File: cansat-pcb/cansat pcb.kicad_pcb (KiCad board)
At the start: 2 copper layers, 63 x 109 mm, 21 parts, among them J1 Conn_01x02_Pin, J4 Conn_01x03_Pin, J5 Conn_01x03_Pin, J6 Conn_01x03_Pin, Q1 AO3400A, Q2 2N3904, Q3 DMG2301L, SW1 SW_DPDT_x2, U3 MPU6050, U5 SGP30

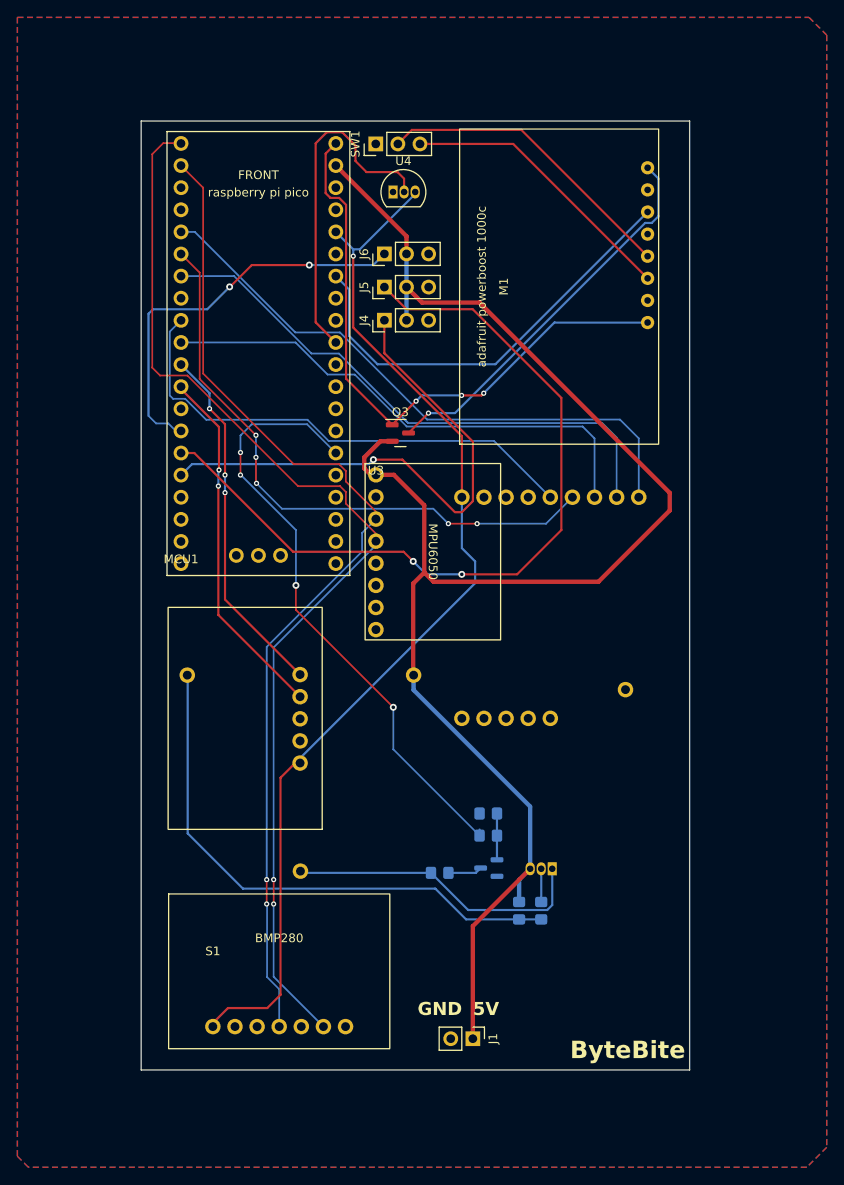
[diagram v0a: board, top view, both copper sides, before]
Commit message: V2
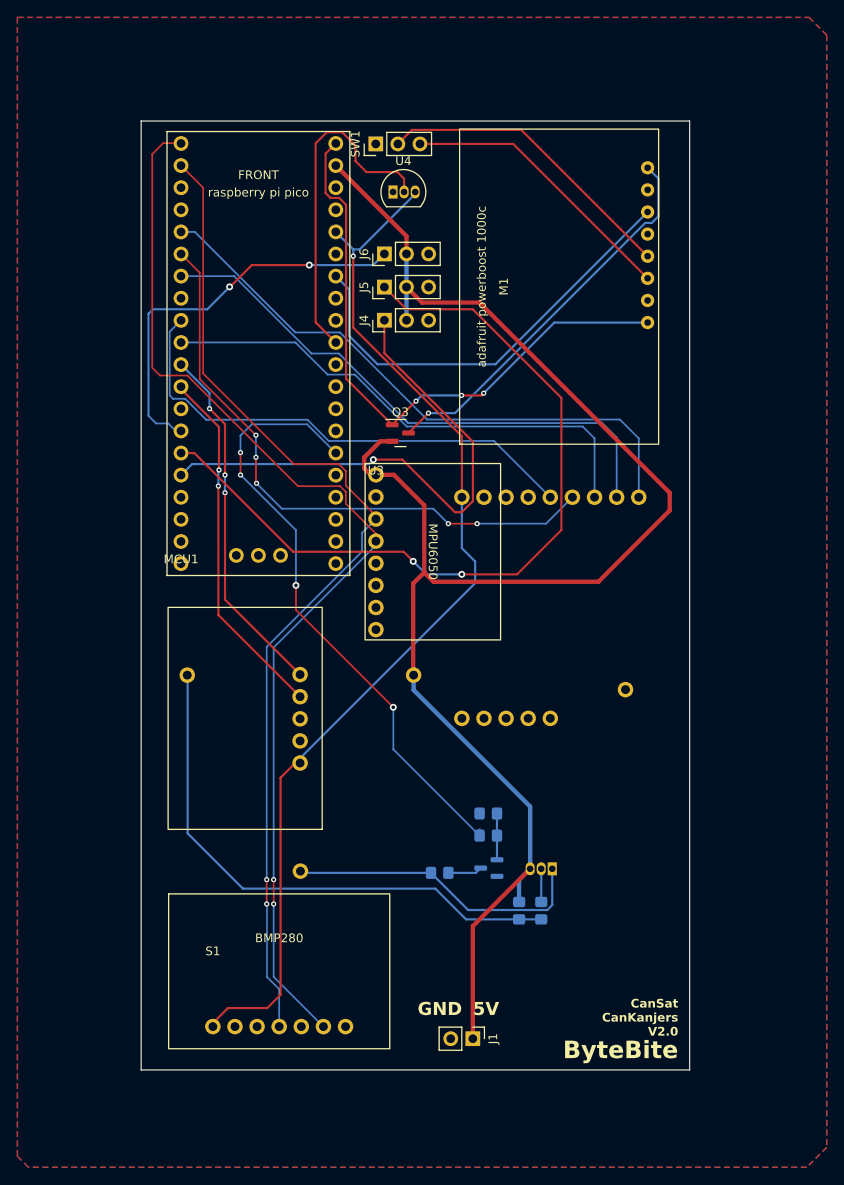
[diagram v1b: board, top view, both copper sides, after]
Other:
- board text added: "CanSat CanKanjers V2.0"
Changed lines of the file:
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@@
   (setup
     (pad_to_mask_clearance 0)
-    (grid_origin 152.14 59.58)
+    (grid_origin 177.54 135.78)
     (pcbplotparams
       (layerselection 0x00010fc_ffffffff)
@@
     (effects (font (size 1.5 1.5) (thickness 0.3) bold) (justify left bottom))
   )
-  (gr_text "ByteBite" (at 181.888 146.714) (layer "F.SilkS")
-    (effects (font (size 2 2) (thickness 0.4) bold))
+  (gr_text "CanSat\nCanKanjers\nV2.0" (at 187.7 145.178) (layer "F.SilkS")
+    (effects (font (size 1 1) (thickness 0.2) bold) (justify right bottom))
+  )
+  (gr_text "ByteBite" (at 187.7 146.714) (layer "F.SilkS")
+    (effects (font (size 2 2) (thickness 0.4) bold) (justify right))
   )
   (segment (start 152.67 78.896) (end 156.006 78.896) (width 0.25) (layer "F.Cu") (net 1))
@@
   (segment (start 158.842346 74.29) (end 180.993 74.29) (width 0.2) (layer "B.Cu") (net 20))
   (segment (start 130.58 52.734) (end 132.161686 52.734) (width 0.2) (layer "B.Cu") (net 20))
-  (segment (start 148.716346 79.404) (end 143.516 79.404) (width 0.2) (layer "F.Cu") (net 22))
-  (segment (start 149.51 80.197654) (end 148.716346 79.404) (width 0.2) (layer "F.Cu") (net 22))
-  (segment (start 149.51 81.404635) (end 152.966865 84.8615) (width 0.2) (layer "F.Cu") (net 22))
-  (segment (start 143.516 79.404) (end 133.12 69.008) (width 0.2) (layer "F.Cu") (net 22))
-  (segment (start 152.966865 84.8615) (end 152.966865 85.72) (width 0.2) (layer "F.Cu") (net 22))
-  (segment (start 149.51 80.197654) (end 149.51 81.404635) (width 0.2) (layer "F.Cu") (net 22))
-  (segment (start 133.12 69.008) (end 133.12 47.654) (width 0.2) (layer "F.Cu") (net 22))
-  (segment (start 133.12 47.654) (end 130.58 45.114) (width 0.2) (layer "F.Cu") (net 22))
+  (segment (start 149.51 81.877317) (end 152.966865 85.334182) (width 0.2) (layer "F.Cu") (net 22))
+  (segment (start 130.58 45.114) (end 133.12 47.654) (width 0.2) (layer "F.Cu") (net 22))
+  (segment (start 133.12 69.008) (end 143.516 79.404) (width 0.2) (layer "F.Cu") (net 22))
+  (segment (start 152.966865 85.334182) (end 152.966865 85.72) (width 0.2) (layer "F.Cu") (net 22))
+  (segment (start 133.12 47.654) (end 133.12 69.008) (width 0.2) (layer "F.Cu") (net 22))
+  (segment (start 148.716346 79.404) (end 149.51 80.197654) (width 0.2) (layer "F.Cu") (net 22))
+  (segment (start 143.516 79.404) (end 148.716346 79.404) (width 0.2) (layer "F.Cu") (net 22))
+  (segment (start 149.51 80.197654) (end 149.51 81.877317) (width 0.2) (layer "F.Cu") (net 22))
   (segment (start 140.418497 129.938) (end 140.418497 127.144) (width 0.2) (layer "F.Cu") (net 22))
   (via (at 140.418497 129.938) (size 0.6) (drill 0.3) (layers "F.Cu" "B.Cu") (net 22))
@@
     )
   )
+  (group "" (id 2326a1ff-ea58-45eb-ac90-ccae38486457)
+    (members
+      74ee758d-d28b-4c85-8a1d-747cfb82e51b
+      9ecb90c8-c273-47ff-8d79-826d2735b5df
+    )
+  )
